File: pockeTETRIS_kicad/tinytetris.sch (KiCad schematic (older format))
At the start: 5 parts

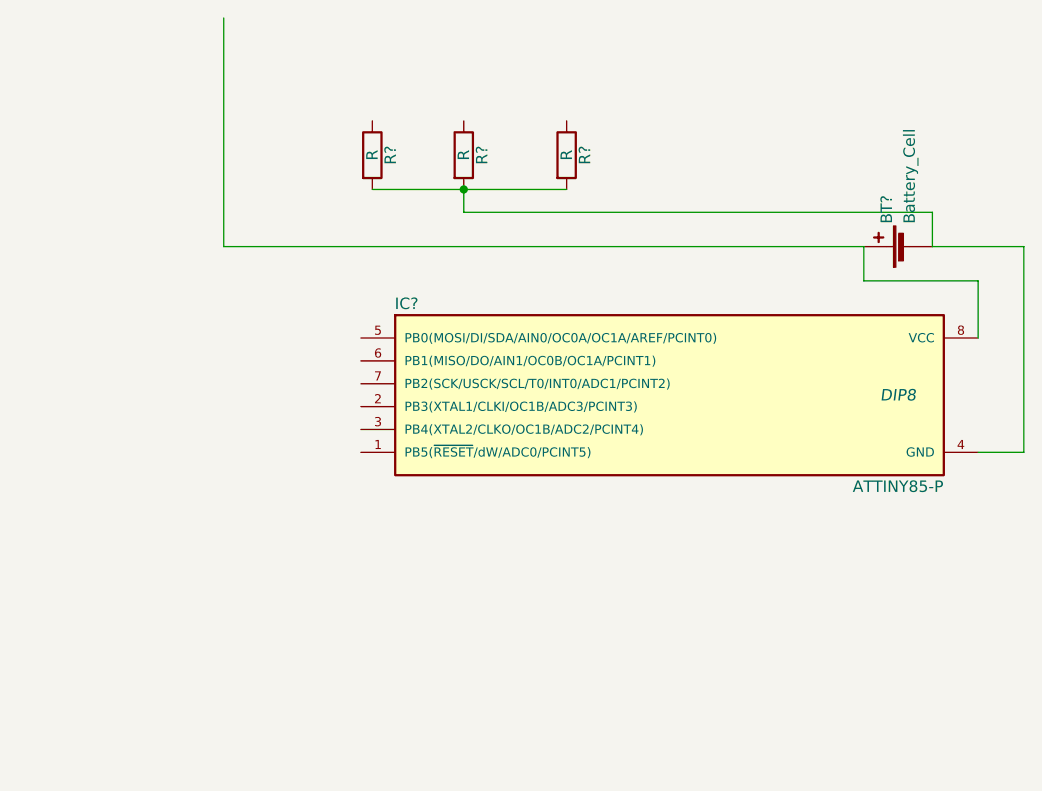
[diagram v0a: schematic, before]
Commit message: Added schematic
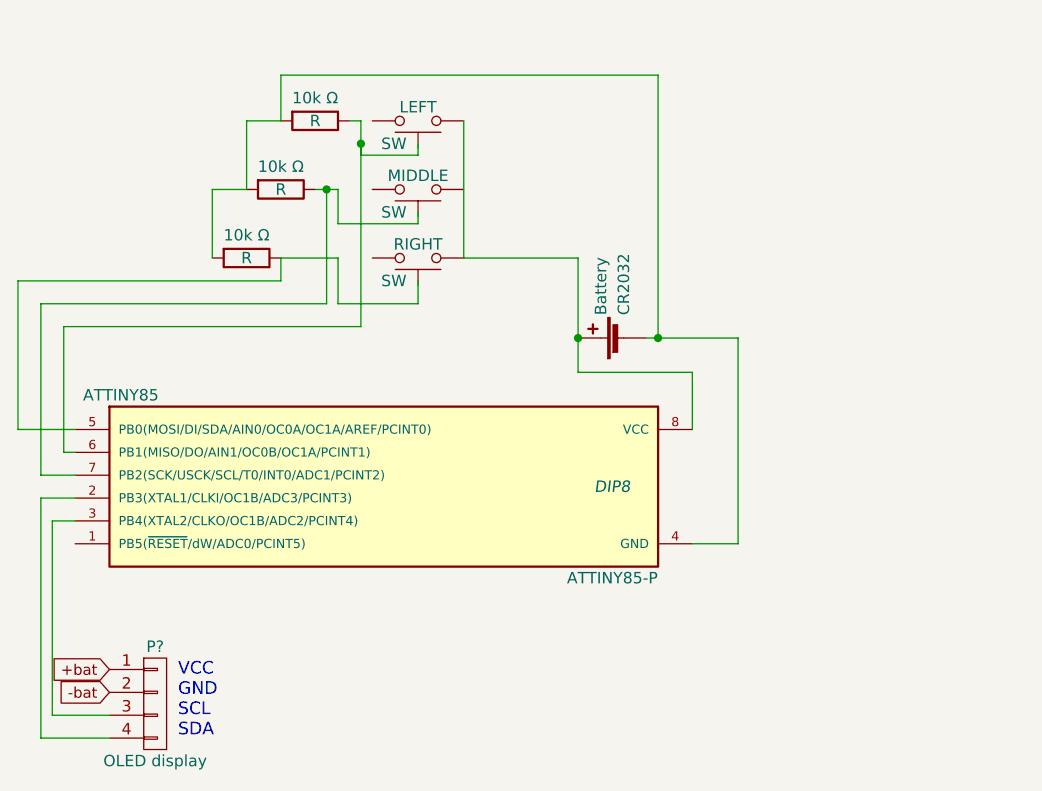
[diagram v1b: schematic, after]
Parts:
- added P?: OLED display, symbol CONN_01X04
- added SW: LEFT, symbol SW_Push
- added SW: MIDDLE, symbol SW_Push
- added SW: RIGHT, symbol SW_Push
- Battery: renamed from BT?; value Battery_Cell -> CR2032
- R: renamed from R?; value R -> 10k Ω
- gave numbers to parts that had none: 1
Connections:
- net labels added: +bat, -bat
- wire segments 12 -> 45
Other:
- note added: "VCC\nGND\nSCL\nSDA"
- moved on the sheet: ATTINY85, Battery, R
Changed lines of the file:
@@
 LIBS:contrib
 LIBS:valves
+LIBS:tinytetris-cache
+LIBS:switches
 EELAYER 25 0
 EELAYER END
@@
 $EndDescr
 $Comp
-L ATTINY85-P IC?
+L ATTINY85-P ATTINY85
 U 1 1 590CE8E1
-P 6950 3800
-F 0 "IC?" H 5800 4200 50  0000 C CNN
-F 1 "ATTINY85-P" H 7950 3400 50  0000 C CNN
-F 2 "DIP8" H 7950 3800 50  0000 C CIN
-F 3 "" H 6950 3800 50  0000 C CNN
-	1    6950 3800
+P 5700 4200
+F 0 "ATTINY85" H 4550 4600 50  0000 C CNN
+F 1 "ATTINY85-P" H 6700 3800 50  0000 C CNN
+F 2 "DIP8" H 6700 4200 50  0000 C CIN
+F 3 "" H 5700 4200 50  0000 C CNN
+	1    5700 4200
 	1    0    0    -1
 $EndComp
 $Comp
-L R R?
+L R R
 U 1 1 590CEA45
-P 6050 2750
-F 0 "R?" V 6130 2750 50  0000 C CNN
-F 1 "R" V 6050 2750 50  0000 C CNN
-F 2 "" V 5980 2750 50  0000 C CNN
-F 3 "" H 6050 2750 50  0000 C CNN
-	1    6050 2750
+P 5100 3200
+F 0 "R" V 5100 3200 50  0000 C CNN
+F 1 "10k Ω" V 5000 3200 50  0000 C CNN
+F 2 "" V 5030 3200 50  0000 C CNN
+F 3 "" H 5100 3200 50  0000 C CNN
+	1    5100 3200
+	0    1    1    0
+$EndComp
+$Comp
+L R R
+U 1 1 590CEAAA
+P 5250 2900
+F 0 "R" V 5250 2900 50  0000 C CNN
+F 1 "10k Ω" V 5150 2900 50  0000 C CNN
+F 2 "" V 5180 2900 50  0000 C CNN
+F 3 "" H 5250 2900 50  0000 C CNN
+	1    5250 2900
+	0    1    1    0
+$EndComp
+$Comp
+L R R
+U 1 1 590CEB9F
+P 5400 2600
+F 0 "R" V 5400 2600 50  0000 C CNN
+F 1 "10k Ω" V 5300 2600 50  0000 C CNN
+F 2 "" V 5330 2600 50  0000 C CNN
+F 3 "" H 5400 2600 50  0000 C CNN
+	1    5400 2600
+	0    1    1    0
+$EndComp
+$Comp
+L Battery_Cell Battery
+U 1 1 590CECF4
+P 6750 3550
+F 0 "Battery" H 6850 3650 50  0000 L CNN
+F 1 "CR2032" H 6850 3550 50  0000 L CNN
+F 2 "" V 6750 3610 50  0000 C CNN
+F 3 "" V 6750 3610 50  0000 C CNN
+	1    6750 3550
+	0    -1   -1   0
+$EndComp
+$Comp
+L CONN_01X04 P?
+U 1 1 59824ECE
+P 4700 5150
+F 0 "P?" H 4700 5400 50  0000 C CNN
+F 1 "OLED display" H 4700 4900 50  0000 C CNN
+F 2 "" H 4700 5150 50  0000 C CNN
+F 3 "" H 4700 5150 50  0000 C CNN
+	1    4700 5150
 	1    0    0    -1
 $EndComp
 $Comp
-L R R?
-U 1 1 590CEAAA
-P 6500 2750
-F 0 "R?" V 6580 2750 50  0000 C CNN
-F 1 "R" V 6500 2750 50  0000 C CNN
-F 2 "" V 6430 2750 50  0000 C CNN
-F 3 "" H 6500 2750 50  0000 C CNN
-	1    6500 2750
-	1    0    0    -1
-$EndComp
-$Comp
-L R R?
-U 1 1 590CEB9F
-P 5650 2750
-F 0 "R?" V 5730 2750 50  0000 C CNN
-F 1 "R" V 5650 2750 50  0000 C CNN
-F 2 "" V 5580 2750 50  0000 C CNN
-F 3 "" H 5650 2750 50  0000 C CNN
-	1    5650 2750
-	1    0    0    -1
-$EndComp
-$Comp
-L Battery_Cell BT?
-U 1 1 590CECF4
-P 8000 3150
-F 0 "BT?" H 8100 3250 50  0000 L CNN
-F 1 "Battery_Cell" H 8100 3150 50  0000 L CNN
-F 2 "" V 8000 3210 50  0000 C CNN
-F 3 "" V 8000 3210 50  0000 C CNN
-	1    8000 3150
-	0    -1   -1   0
-$EndComp
-Wire Wire Line
-	5650 2900 6500 2900
-Connection ~ 6050 2900
-Wire Wire Line
-	6050 2900 6050 3000
-Wire Wire Line
-	6050 3000 8100 3000
-Wire Wire Line
-	8100 3000 8100 3150
-Wire Wire Line
-	8100 3150 8500 3150
-Wire Wire Line
-	8500 3150 8500 4050
-Wire Wire Line
-	8500 4050 8300 4050
-Wire Wire Line
-	8300 3300 8300 3550
-Wire Wire Line
-	7800 3300 8300 3300
-Wire Wire Line
-	7800 3300 7800 3150
-Wire Wire Line
-	7800 3150 5000 3150
-Wire Wire Line
-	5000 3150 5000 2150
+L SW_Push SW
+U 1 1 598FDC40
+P 5850 2900
+F 0 "SW" H 5900 3000 50  0000 L CNN
+F 1 "MIDDLE" H 5850 2840 50  0000 C CNN
+F 2 "" H 5850 3100 50  0000 C CNN
+F 3 "" H 5850 3100 50  0000 C CNN
+	1    5850 2900
+	-1   0    0    1
+$EndComp
+$Comp
+L SW_Push SW
+U 1 1 598FDC85
+P 5850 3200
+F 0 "SW" H 5900 3300 50  0000 L CNN
+F 1 "RIGHT" H 5850 3140 50  0000 C CNN
+F 2 "" H 5850 3400 50  0000 C CNN
+F 3 "" H 5850 3400 50  0000 C CNN
+	1    5850 3200
+	-1   0    0    1
+$EndComp
+$Comp
+L SW_Push SW
+U 1 1 598FDBAF
+P 5850 2600
+F 0 "SW" H 5900 2700 50  0000 L CNN
+F 1 "LEFT" H 5850 2540 50  0000 C CNN
+F 2 "" H 5850 2800 50  0000 C CNN
+F 3 "" H 5850 2800 50  0000 C CNN
+	1    5850 2600
+	-1   0    0    1
+$EndComp
+Wire Wire Line
+	6850 3550 7250 3550
+Wire Wire Line
+	7250 3550 7250 4450
+Wire Wire Line
+	7250 4450 7050 4450
+Wire Wire Line
+	7050 3700 7050 3950
+Wire Wire Line
+	6550 3700 7050 3700
+Connection ~ 6550 3550
+Wire Wire Line
+	6550 3200 6550 3700
+Wire Wire Line
+	6550 3200 6050 3200
+Wire Wire Line
+	6050 3200 6050 2600
+Wire Wire Line
+	5250 2400 6900 2400
+Wire Wire Line
+	6900 2400 6900 3550
+Connection ~ 6900 3550
+Wire Wire Line
+	5250 2400 5250 2600
+Wire Wire Line
+	5250 2600 5100 2600
+Wire Wire Line
+	5100 2600 5100 2900
+Wire Wire Line
+	5100 2900 4950 2900
+Wire Wire Line
+	4950 2900 4950 3200
+Wire Wire Line
+	5250 3200 5250 3300
+Wire Wire Line
+	5250 3300 4100 3300
+Wire Wire Line
+	4100 3300 4100 3950
+Wire Wire Line
+	4100 3950 4350 3950
+Wire Wire Line
+	5450 2900 5450 3400
+Wire Wire Line
+	5450 3400 4200 3400
+Wire Wire Line
+	4200 3400 4200 4150
+Wire Wire Line
+	4200 4150 4350 4150
+Wire Wire Line
+	5600 3500 4300 3500
+Wire Wire Line
+	4300 3500 4300 4050
+Wire Wire Line
+	4300 4050 4350 4050
+Wire Wire Line
+	4500 5200 4250 5200
+Wire Wire Line
+	4250 5200 4250 4350
+Wire Wire Line
+	4250 4350 4350 4350
+Wire Wire Line
+	4200 5300 4500 5300
+Wire Wire Line
+	4200 5300 4200 4250
+Wire Wire Line
+	4200 4250 4350 4250
+Text GLabel 4500 5100 0    47   Input ~ 0
+-bat
+Text GLabel 4500 5000 0    47   Input ~ 0
++bat
+Text Notes 4800 5300 0    55   ~ 0
+VCC\nGND\nSCL\nSDA
+Wire Wire Line
+	5850 3300 5850 3400
+Wire Wire Line
+	5850 3000 5850 3050
+Wire Wire Line
+	5850 2700 5850 2750
+Wire Wire Line
+	5850 2750 5600 2750
+Wire Wire Line
+	5600 2750 5600 2600
+Wire Wire Line
+	5600 2600 5550 2600
+Wire Wire Line
+	5600 3500 5600 2700
+Connection ~ 5600 2700
+Wire Wire Line
+	5850 3050 5500 3050
+Wire Wire Line
+	5500 3050 5500 2900
+Wire Wire Line
+	5500 2900 5400 2900
+Connection ~ 5450 2900
+Wire Wire Line
+	5850 3400 5500 3400
+Wire Wire Line
+	5500 3400 5500 3200
+Wire Wire Line
+	5500 3200 5250 3200
 $EndSCHEMATC
